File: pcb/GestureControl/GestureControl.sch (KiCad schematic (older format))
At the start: 72 parts, among them J1 Conn_01x04_I2I-LCD, J2 BATT, J3 Conn_01x08, J4 Conn_01x06, J5 Conn_01x10, J6 Conn_01x08, SW1 SW1, SW2 SW2, U1 AP5100_3.3, U2 AP5100_3.3

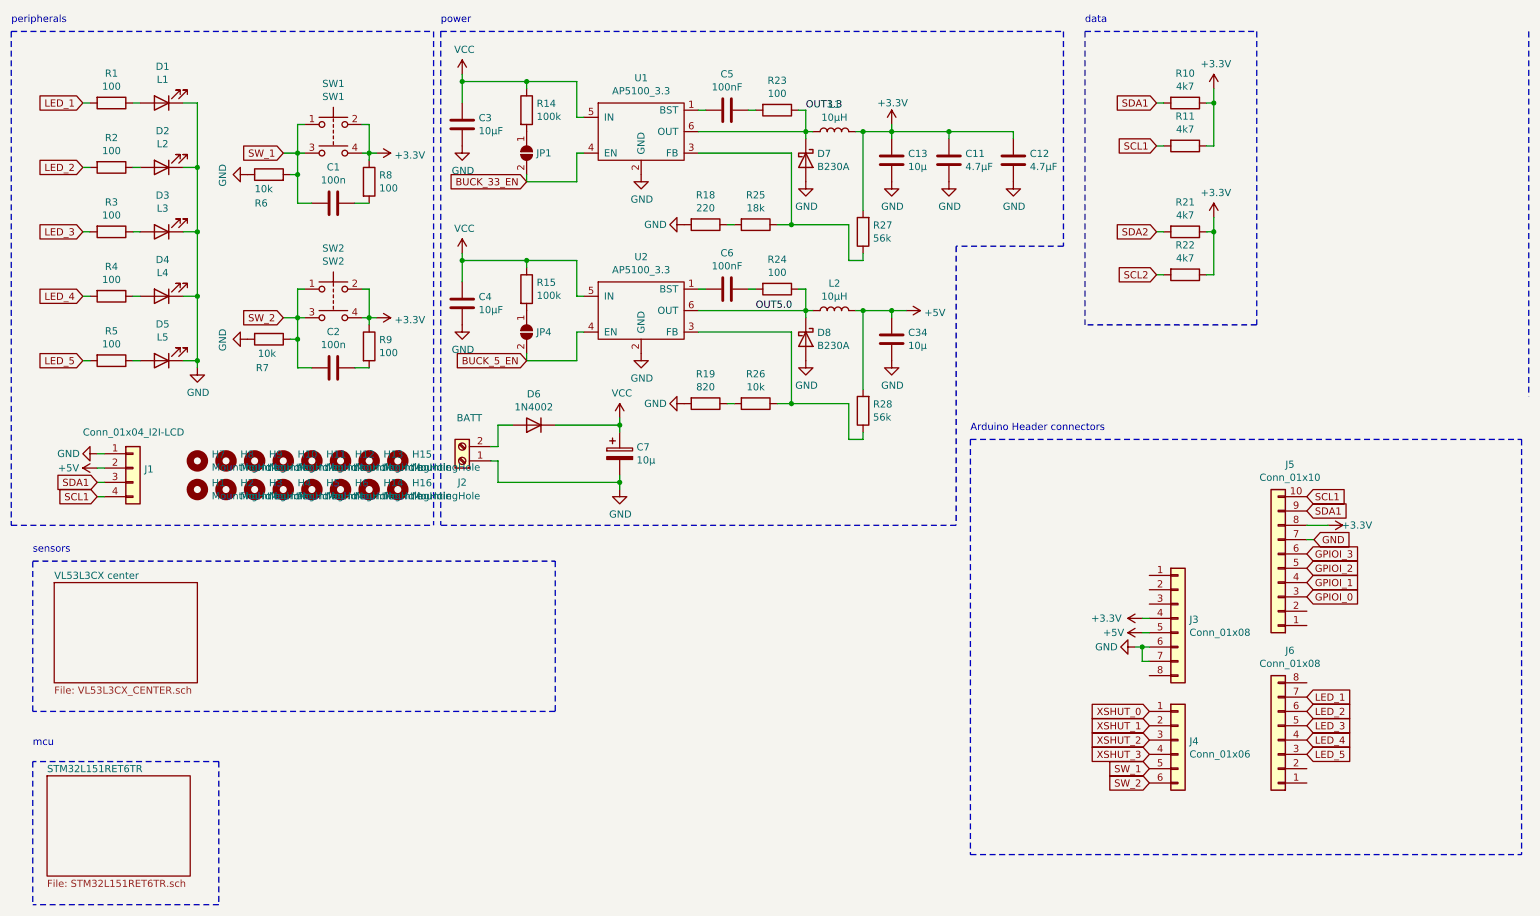
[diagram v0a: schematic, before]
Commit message: cleanup PCB V0.1
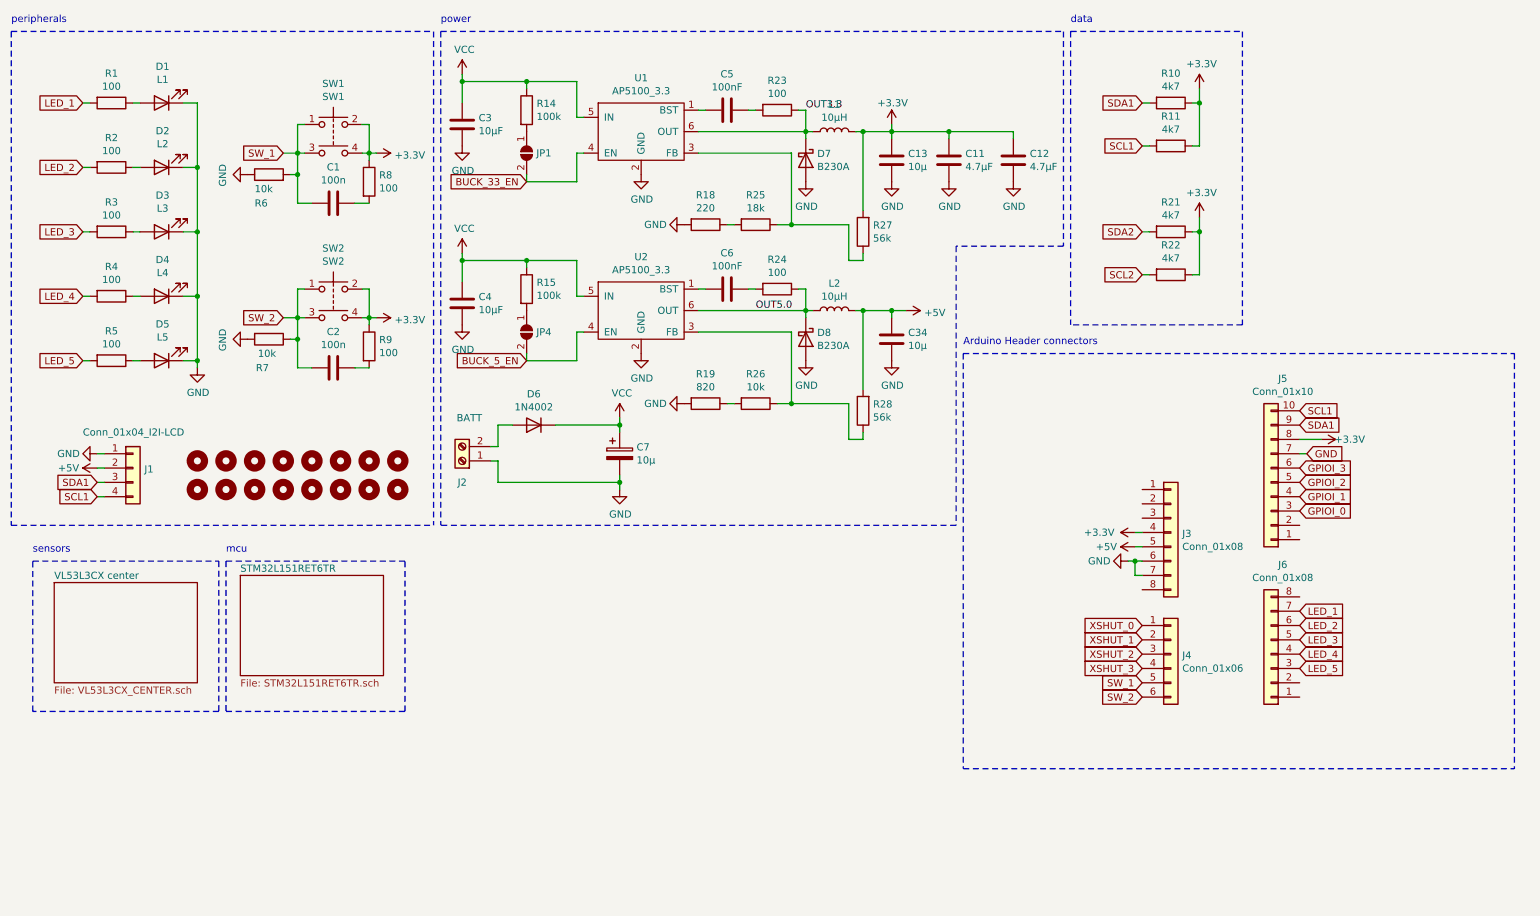
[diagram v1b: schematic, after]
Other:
- moved on the sheet: J3, J4, J5, J6, R10, R11, R21, R22
